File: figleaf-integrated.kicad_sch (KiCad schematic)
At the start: 63 parts, among them J1 UDB, J2 HRO_TYPE-C-31-M-14, J3 Battery, J9 TC2030_SWD, Q2 2N7002, SW1 PWR, SW2 RST, U1 SRV05-4, U10 MAX17048, U3 BQ24075, U8 nRF52840_moko_mk08

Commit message: progress + add jst conn
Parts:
- J3: footprint PCM_marbastlib-various:Molex_Pico-EZmate_78171-0002_1x02-1MP_P1.20mm_Vertical -> Connector_JST:JST_SH_SM02B-SRSS-TB_1x02-1MP_P1.00mm_Horizontal
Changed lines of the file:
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@@
 			)
 		)
-		(property "Footprint" "PCM_marbastlib-various:Molex_Pico-EZmate_78171-0002_1x02-1MP_P1.20mm_Vertical"
+		(property "Footprint" "Connector_JST:JST_SH_SM02B-SRSS-TB_1x02-1MP_P1.00mm_Horizontal"
 			(at 236.22 57.15 0)
 			(effects

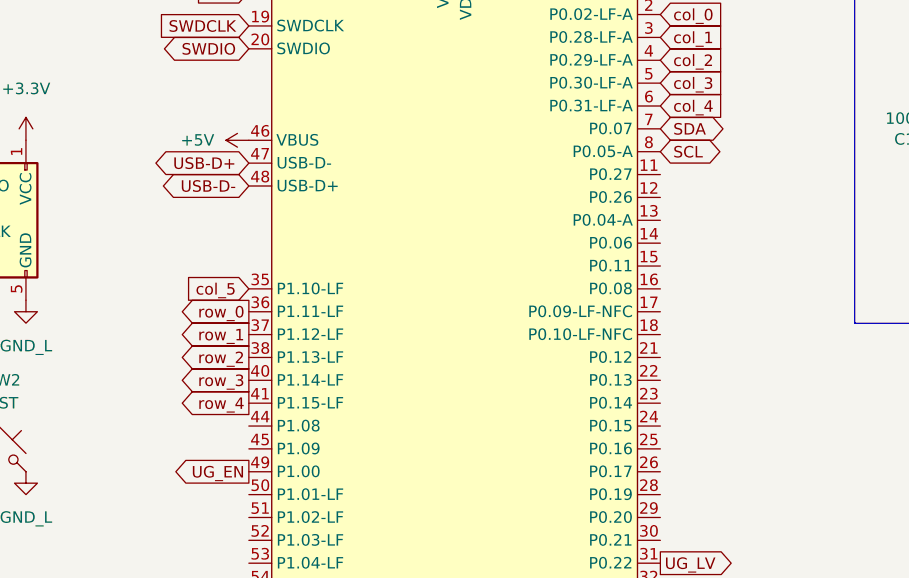
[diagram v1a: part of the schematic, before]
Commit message: Add matrix
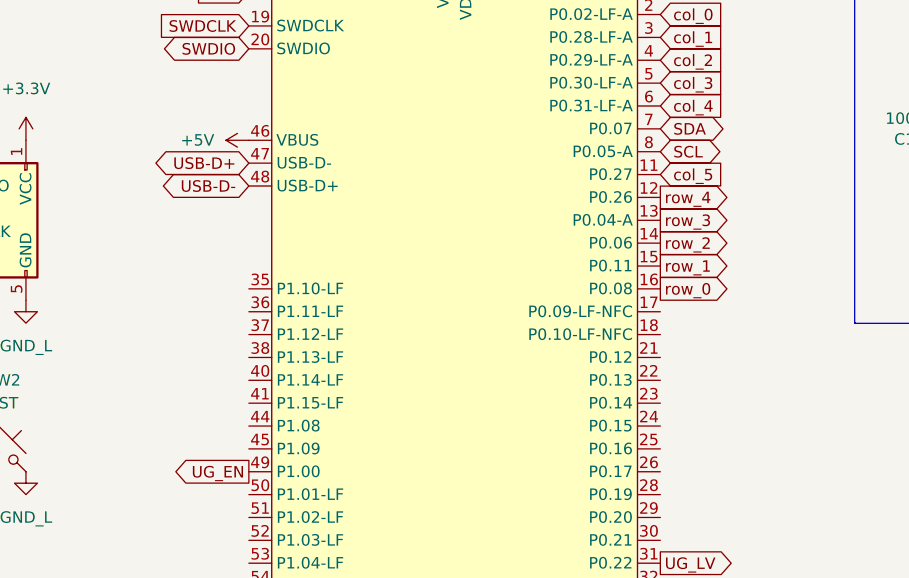
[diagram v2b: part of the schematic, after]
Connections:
- net col_5: now also U8.11 (P0.27); no longer U8.35 (P1.10-LF)
- net row_0: now also U8.16 (P0.08); no longer U8.36 (P1.11-LF)
- net row_1: now also U8.15 (P0.11); no longer U8.37 (P1.12-LF)
- net row_2: now also U8.14 (P0.06); no longer U8.38 (P1.13-LF)
- net row_3: now also U8.13 (P0.04-A); no longer U8.40 (P1.14-LF)
- net row_4: now also U8.12 (P0.26); no longer U8.41 (P1.15-LF)

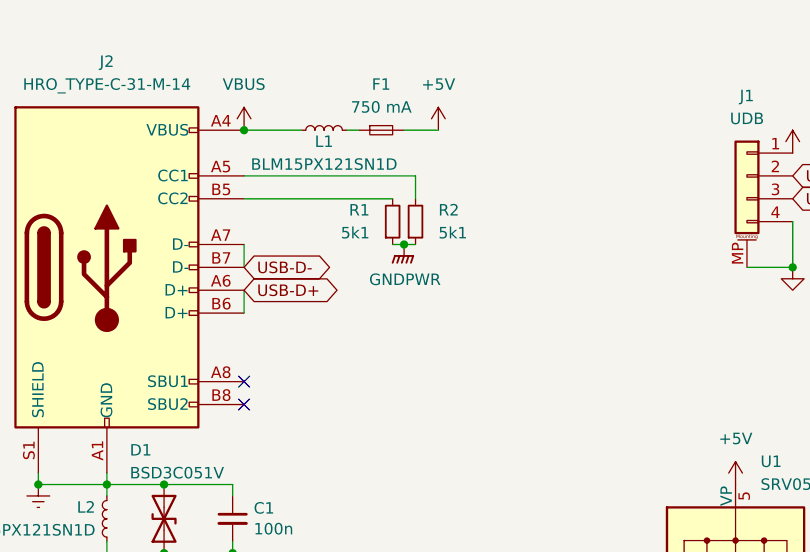
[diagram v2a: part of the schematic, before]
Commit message: tracing progress
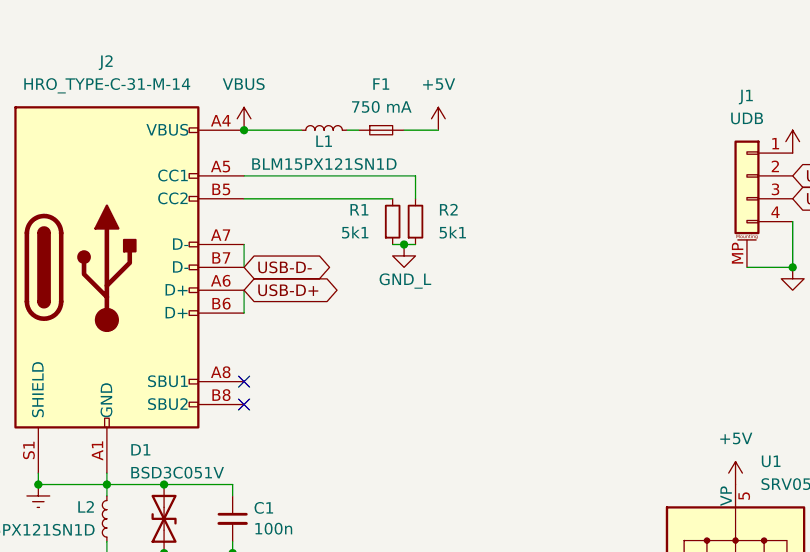
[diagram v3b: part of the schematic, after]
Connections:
- net GNDPWR is gone; now on net GND_L: R1.1, R2.1
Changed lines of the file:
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@@
 	)
 	(symbol
-		(lib_id "power:GNDPWR")
+		(lib_id "power:GND")
 		(at 67.31 41.91 0)
 		(unit 1)
@@
 			)
 		)
-		(property "Value" "GNDPWR"
+		(property "Value" "GND_L"
 			(at 67.4116 45.8216 0)
 			(effects
@@
 		)
 		(property "Footprint" ""
-			(at 67.31 43.18 0)
+			(at 67.31 41.91 0)
 			(effects
 				(font
@@
 		)
 		(property "Datasheet" ""
-			(at 67.31 43.18 0)
+			(at 67.31 41.91 0)
 			(effects
 				(font
@@
 			)
 		)
-		(property "Description" "Power symbol creates a global label with name \"GNDPWR\" , global ground"
+		(property "Description" "Power symbol creates a global label with name \"GND\" , ground"
 			(at 67.31 41.91 0)
 			(effects
